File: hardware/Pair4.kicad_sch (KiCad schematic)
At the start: 10 parts, among them IC4 TPS2HCS08AQPWPRQ1, J15 Conn_01x02, J7 Conn_01x02

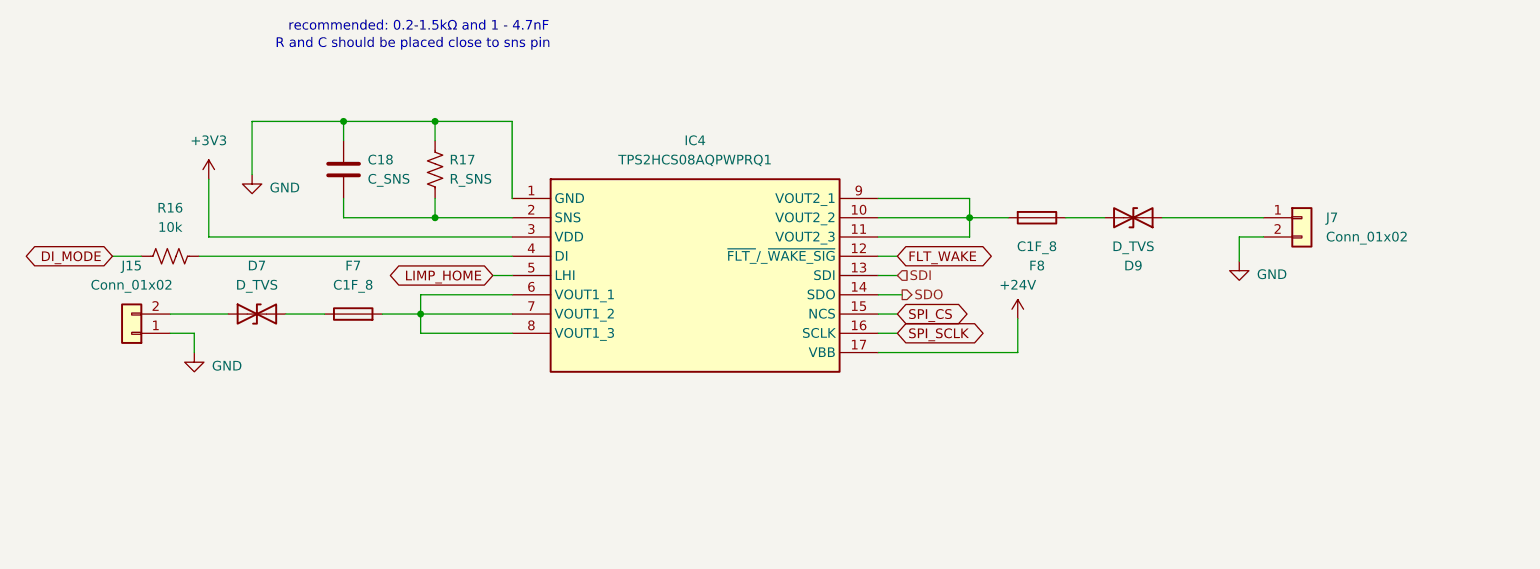
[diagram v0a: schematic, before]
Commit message: aesthetic added
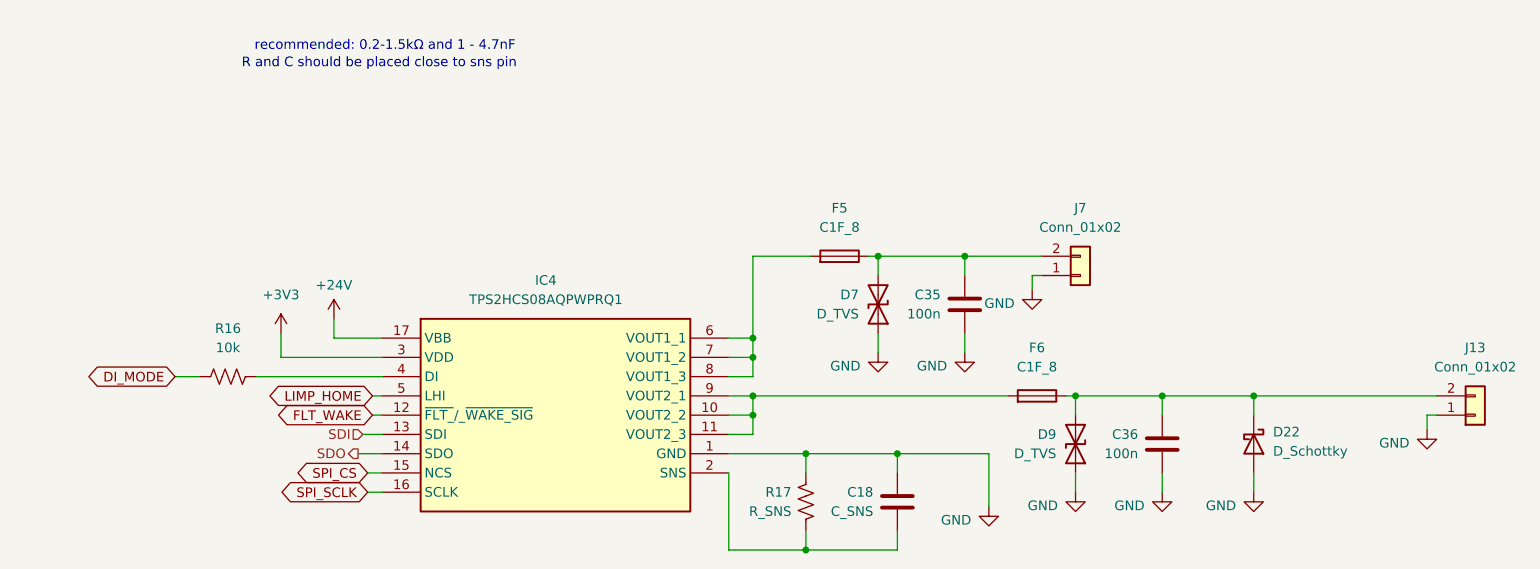
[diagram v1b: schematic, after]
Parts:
- removed F7, F8: C1F_8, Fuse:Fuse_1206_3216Metric, symbol PowerDistributionUnitLib:C1F_8
- removed J15: Conn_01x02, symbol Connector_Generic:Conn_01x02
- added C35, C36: 100n, symbol Device:C
- added D22: D_Schottky, symbol Device:D_Schottky
- added F5, F6: C1F_8, Fuse:Fuse_1206_3216Metric, symbol PowerDistributionUnitLib:C1F_8
- added J13: Conn_01x02, symbol Connector_Generic:Conn_01x02
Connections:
- net GND: now also D7.1 (A1), D9.1 (A1), J7.1 (Pin_1), C35.1, C36.1, D22.2 (A), J13.1 (Pin_1); no longer J7.2 (Pin_2)
- net at D9.2 (A2): now also C36.2, D22.1 (K), F6.1, J13.2 (Pin_2)
- net at IC4.10 (VOUT2_2), IC4.11 (VOUT2_3), IC4.9 (VOUT2_1): now also F6.2
- net at IC4.6 (VOUT1_1), IC4.7 (VOUT1_2), IC4.8 (VOUT1_3): now also F5.2
- net at D7.2 (A2): now also J7.2 (Pin_2), C35.2, F5.1
